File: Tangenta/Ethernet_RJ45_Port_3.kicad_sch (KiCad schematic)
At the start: 2 parts, among them J7 HY911130A

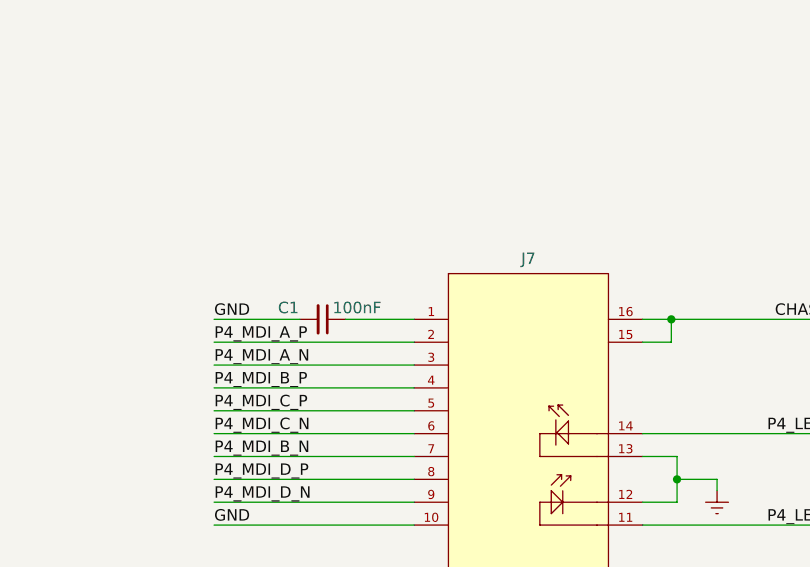
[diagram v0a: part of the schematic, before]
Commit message: initialize branch
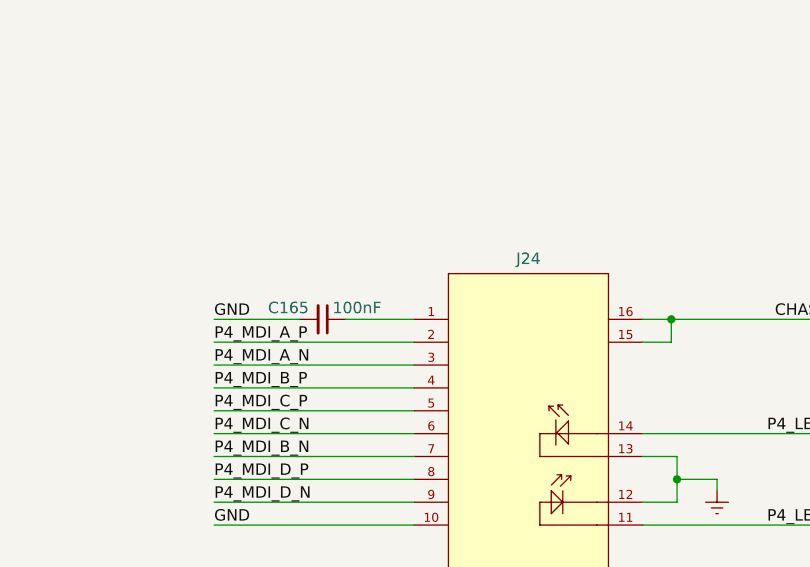
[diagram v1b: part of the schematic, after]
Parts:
- renumbered C1 to C165, J7 to J24
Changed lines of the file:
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@@
   (symbol (lib_id "power:GNDREF") (at 168.275 89.535 0) (mirror y) (unit 1)
     (in_bom yes) (on_board yes) (dnp no) (fields_autoplaced)
-    (property "Reference" "#PWR013" (at 168.275 95.885 0)
+    (property "Reference" "#PWR078" (at 168.275 95.885 0)
       (effects (font (size 1.27 1.27)) hide)
     )
@@
     (instances
       (project "Tangenta"
-        (path "/358d1bcf-7599-4352-8c4d-baa18a5f09e6/d6c05402-162e-441f-bed8-be7996260fb4"
-          (reference "#PWR013") (unit 1)
-        )
-        (path "/358d1bcf-7599-4352-8c4d-baa18a5f09e6/9b1f6f94-444c-4c59-8de9-290bde336856"
-          (reference "#PWR050") (unit 1)
-        )
-        (path "/358d1bcf-7599-4352-8c4d-baa18a5f09e6/9b1f6f94-444c-4c59-8de9-290bde336856/04648235-6c5e-4915-ab80-8fea22048f3c"
-          (reference "#PWR050") (unit 1)
-        )
-        (path "/358d1bcf-7599-4352-8c4d-baa18a5f09e6/2bb52479-7b35-496d-9807-27e706c6ef7b"
-          (reference "#PWR059") (unit 1)
-        )
-        (path "/358d1bcf-7599-4352-8c4d-baa18a5f09e6/2bb52479-7b35-496d-9807-27e706c6ef7b/c653b84e-94ee-4be9-b47c-8c767f88973e"
-          (reference "#PWR059") (unit 1)
-        )
-        (path "/358d1bcf-7599-4352-8c4d-baa18a5f09e6/2bb52479-7b35-496d-9807-27e706c6ef7b/107b1895-3302-473d-bd1c-b123cf003d25"
-          (reference "#PWR069") (unit 1)
-        )
         (path "/358d1bcf-7599-4352-8c4d-baa18a5f09e6/2bb52479-7b35-496d-9807-27e706c6ef7b/5dd23ea2-ad33-4f2c-a45e-3d59d95f0b2c"
           (reference "#PWR078") (unit 1)
@@
   (symbol (lib_id "power:GNDREF") (at 25.4 24.13 270) (mirror x) (unit 1)
     (in_bom yes) (on_board yes) (dnp no) (fields_autoplaced)
-    (property "Reference" "#PWR013" (at 19.05 24.13 0)
+    (property "Reference" "#PWR077" (at 19.05 24.13 0)
       (effects (font (size 1.27 1.27)) hide)
     )
@@
     (instances
       (project "Tangenta"
-        (path "/358d1bcf-7599-4352-8c4d-baa18a5f09e6/d6c05402-162e-441f-bed8-be7996260fb4"
-          (reference "#PWR013") (unit 1)
-        )
-        (path "/358d1bcf-7599-4352-8c4d-baa18a5f09e6/9b1f6f94-444c-4c59-8de9-290bde336856"
-          (reference "#PWR050") (unit 1)
-        )
-        (path "/358d1bcf-7599-4352-8c4d-baa18a5f09e6/9b1f6f94-444c-4c59-8de9-290bde336856/04648235-6c5e-4915-ab80-8fea22048f3c"
-          (reference "#PWR050") (unit 1)
-        )
-        (path "/358d1bcf-7599-4352-8c4d-baa18a5f09e6/2bb52479-7b35-496d-9807-27e706c6ef7b"
-          (reference "#PWR059") (unit 1)
-        )
-        (path "/358d1bcf-7599-4352-8c4d-baa18a5f09e6/2bb52479-7b35-496d-9807-27e706c6ef7b/c653b84e-94ee-4be9-b47c-8c767f88973e"
-          (reference "#PWR059") (unit 1)
-        )
         (path "/358d1bcf-7599-4352-8c4d-baa18a5f09e6/2bb52479-7b35-496d-9807-27e706c6ef7b/5dd23ea2-ad33-4f2c-a45e-3d59d95f0b2c"
           (reference "#PWR077") (unit 1)
@@
   (symbol (lib_id "CholaSymbolsPrjLib:C_Small") (at 124.46 70.485 270) (unit 1)
     (in_bom yes) (on_board yes) (dnp no)
-    (property "Reference" "C1" (at 120.65 69.215 90)
+    (property "Reference" "C165" (at 120.65 69.215 90)
       (effects (font (size 1.27 1.27)))
     )
@@
     (instances
       (project "Tangenta"
-        (path "/358d1bcf-7599-4352-8c4d-baa18a5f09e6/8215796b-9611-4f43-bcc5-319f8414b8a6"
-          (reference "C1") (unit 1)
-        )
-        (path "/358d1bcf-7599-4352-8c4d-baa18a5f09e6/d6c05402-162e-441f-bed8-be7996260fb4"
-          (reference "C9") (unit 1)
-        )
-        (path "/358d1bcf-7599-4352-8c4d-baa18a5f09e6/b1871a4d-6a35-44e2-a9a2-9a4af684371d"
-          (reference "C40") (unit 1)
-        )
-        (path "/358d1bcf-7599-4352-8c4d-baa18a5f09e6/6a8c68b5-4a7d-449e-86f6-34ced6d1cb55"
-          (reference "C81") (unit 1)
-        )
-        (path "/358d1bcf-7599-4352-8c4d-baa18a5f09e6/9b1f6f94-444c-4c59-8de9-290bde336856/04648235-6c5e-4915-ab80-8fea22048f3c"
-          (reference "C98") (unit 1)
-        )
-        (path "/358d1bcf-7599-4352-8c4d-baa18a5f09e6/2bb52479-7b35-496d-9807-27e706c6ef7b"
-          (reference "C157") (unit 1)
-        )
-        (path "/358d1bcf-7599-4352-8c4d-baa18a5f09e6/2bb52479-7b35-496d-9807-27e706c6ef7b/c653b84e-94ee-4be9-b47c-8c767f88973e"
-          (reference "C170") (unit 1)
-        )
-        (path "/358d1bcf-7599-4352-8c4d-baa18a5f09e6/2bb52479-7b35-496d-9807-27e706c6ef7b/8c8da075-62e5-4ec4-9abc-b27287749d5c"
-          (reference "C164") (unit 1)
-        )
-        (path "/358d1bcf-7599-4352-8c4d-baa18a5f09e6/2bb52479-7b35-496d-9807-27e706c6ef7b/107b1895-3302-473d-bd1c-b123cf003d25"
-          (reference "C173") (unit 1)
-        )
         (path "/358d1bcf-7599-4352-8c4d-baa18a5f09e6/2bb52479-7b35-496d-9807-27e706c6ef7b/5dd23ea2-ad33-4f2c-a45e-3d59d95f0b2c"
           (reference "C165") (unit 1)
@@
   (symbol (lib_id "CholaSymbolsPrjLib:HY911130A") (at 147.32 81.915 0) (unit 1)
     (in_bom yes) (on_board yes) (dnp no)
-    (property "Reference" "J7" (at 147.32 63.754 0)
+    (property "Reference" "J24" (at 147.32 63.754 0)
       (effects (font (size 1.27 1.27)))
     )
@@
     (instances
       (project "Tangenta"
-        (path "/358d1bcf-7599-4352-8c4d-baa18a5f09e6/2bb52479-7b35-496d-9807-27e706c6ef7b"
-          (reference "J7") (unit 1)
-        )
         (path "/358d1bcf-7599-4352-8c4d-baa18a5f09e6/2bb52479-7b35-496d-9807-27e706c6ef7b/5dd23ea2-ad33-4f2c-a45e-3d59d95f0b2c"
           (reference "J24") (unit 1)

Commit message: J6-J8,J22-J25,S1,U21
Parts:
- J24: footprint RJ45_MAGJACK:RJ45_MAGJACK_HY911130A -> CholaFootprintsPrjLib:RJ45_MAGJACK_HY911130A
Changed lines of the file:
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@@
       (effects (font (size 1.27 1.27)))
     )
-    (property "Footprint" "RJ45_MAGJACK:RJ45_MAGJACK_HY911130A" (at 168.91 104.775 0)
+    (property "Footprint" "CholaFootprintsPrjLib:RJ45_MAGJACK_HY911130A" (at 168.91 104.775 0)
       (effects (font (size 1.27 1.27) italic) hide)
     )
